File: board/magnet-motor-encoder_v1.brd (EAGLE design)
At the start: 22 x 22 mm, 12 parts, among them IC1 AS5045B

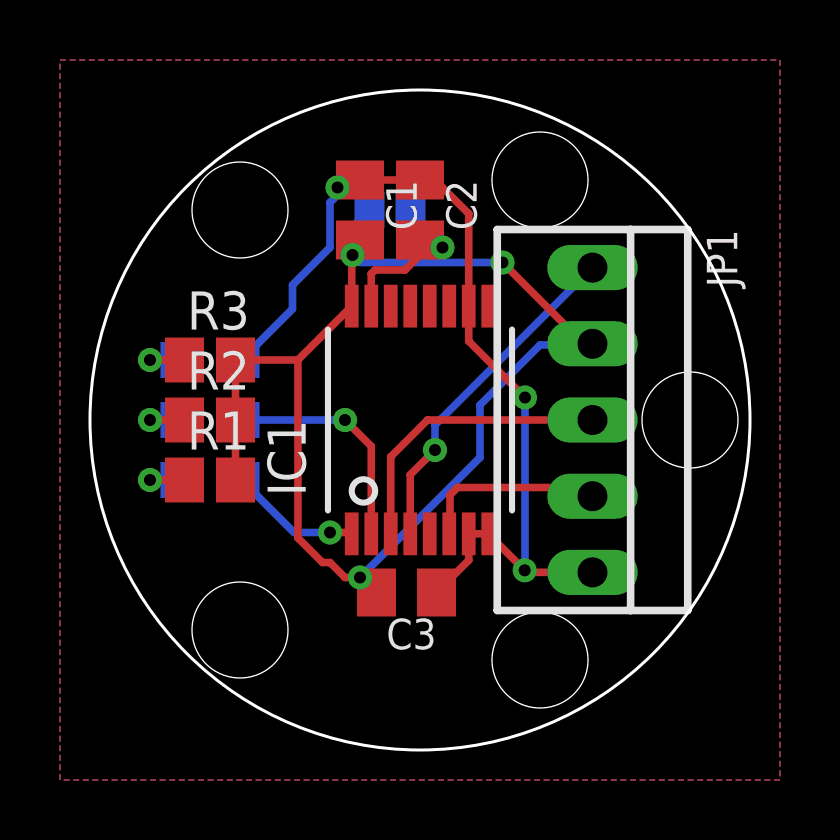
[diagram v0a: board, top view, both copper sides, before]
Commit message: board layout and silkscreen
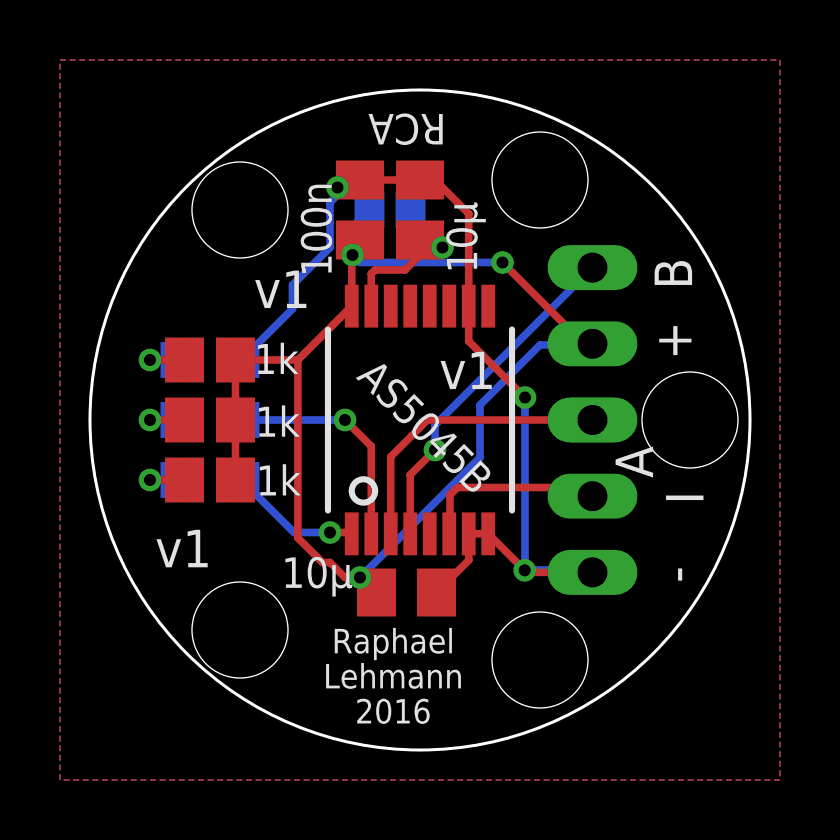
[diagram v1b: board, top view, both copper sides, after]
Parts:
- LED_BLUE: value BLUE -> POWER
- LED_RED: value RED -> DEC
- LED_YELLOW: value YELLOW -> INC
- R1, R2: value 330 -> 1k
- SJ1: value 5V? -> 3V3?
- flipped JP1 to the bottom
- renumbered LED1 to LED_YELLOW, LED2 to LED_RED, LED3 to LED_BLUE
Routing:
- net GND: track 32.0 -> 34.3 mm
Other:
- board text added: "+"
- board text added: "-"
- board text added: "A"
- board text added: "B"
- board text added: "BLUE"
- board text added: "I"
- board text added: "INC DEC POWER"
- board text added: "LEDs 2mA"
- board text added: "Magnet Motor Encoder"
- board text added: "RCA"
- board text added: "RED"
- board text added: "Raphael Lehmann 2016"
- board text added: "Solder"
- board text added: "YELLOW"
- board text added: "for 3V3"
- board text added: "low current"
- board text added: "v1"
